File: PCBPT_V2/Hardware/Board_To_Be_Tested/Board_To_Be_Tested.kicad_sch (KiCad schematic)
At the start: 20 parts, among them U1 SHT15, U2 MOUDLE-SEEEDUINO-XIAO

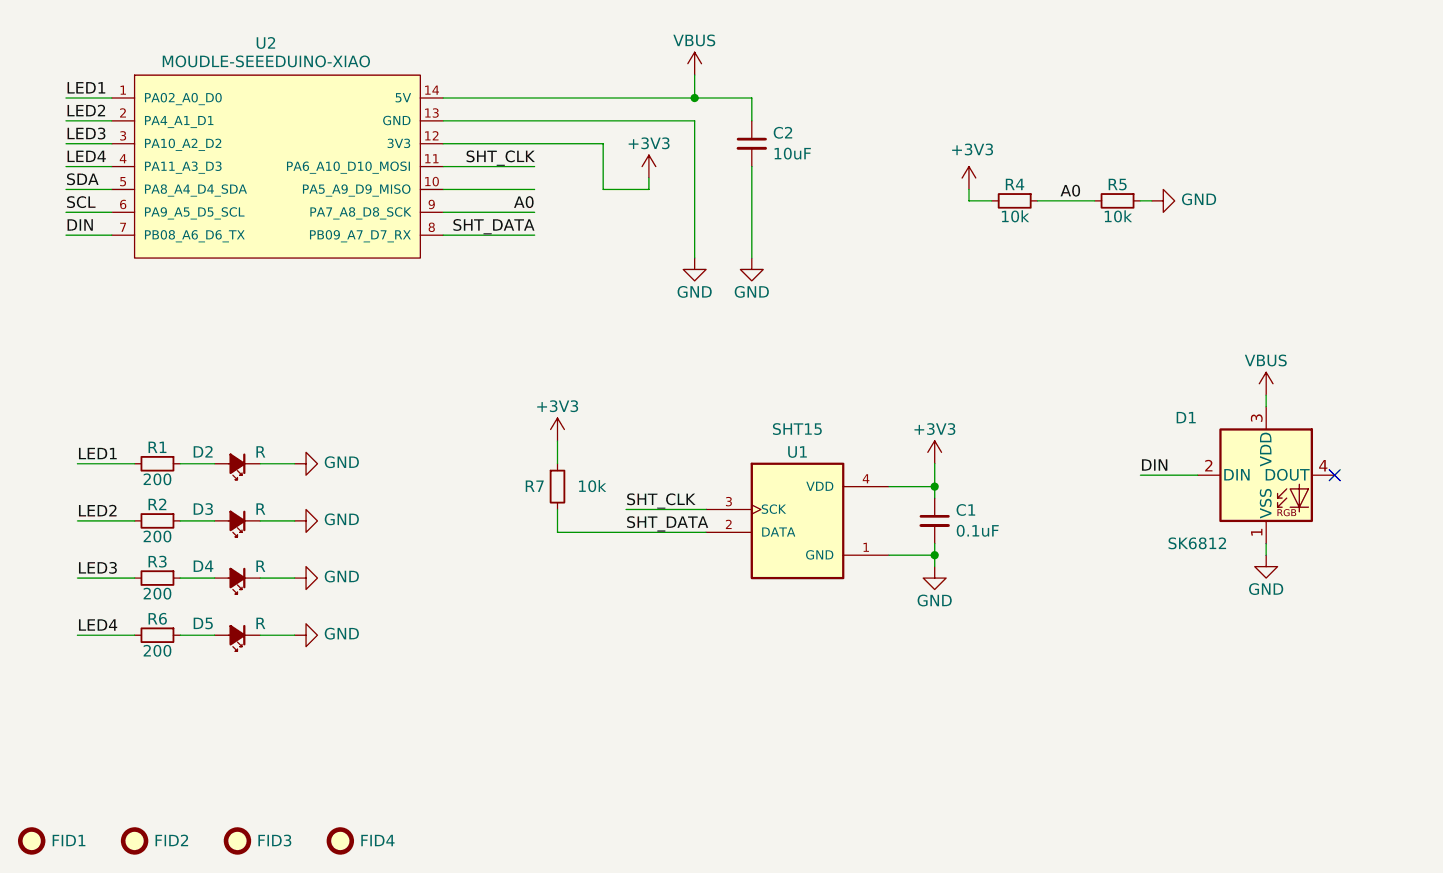
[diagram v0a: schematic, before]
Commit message: udated by FZ
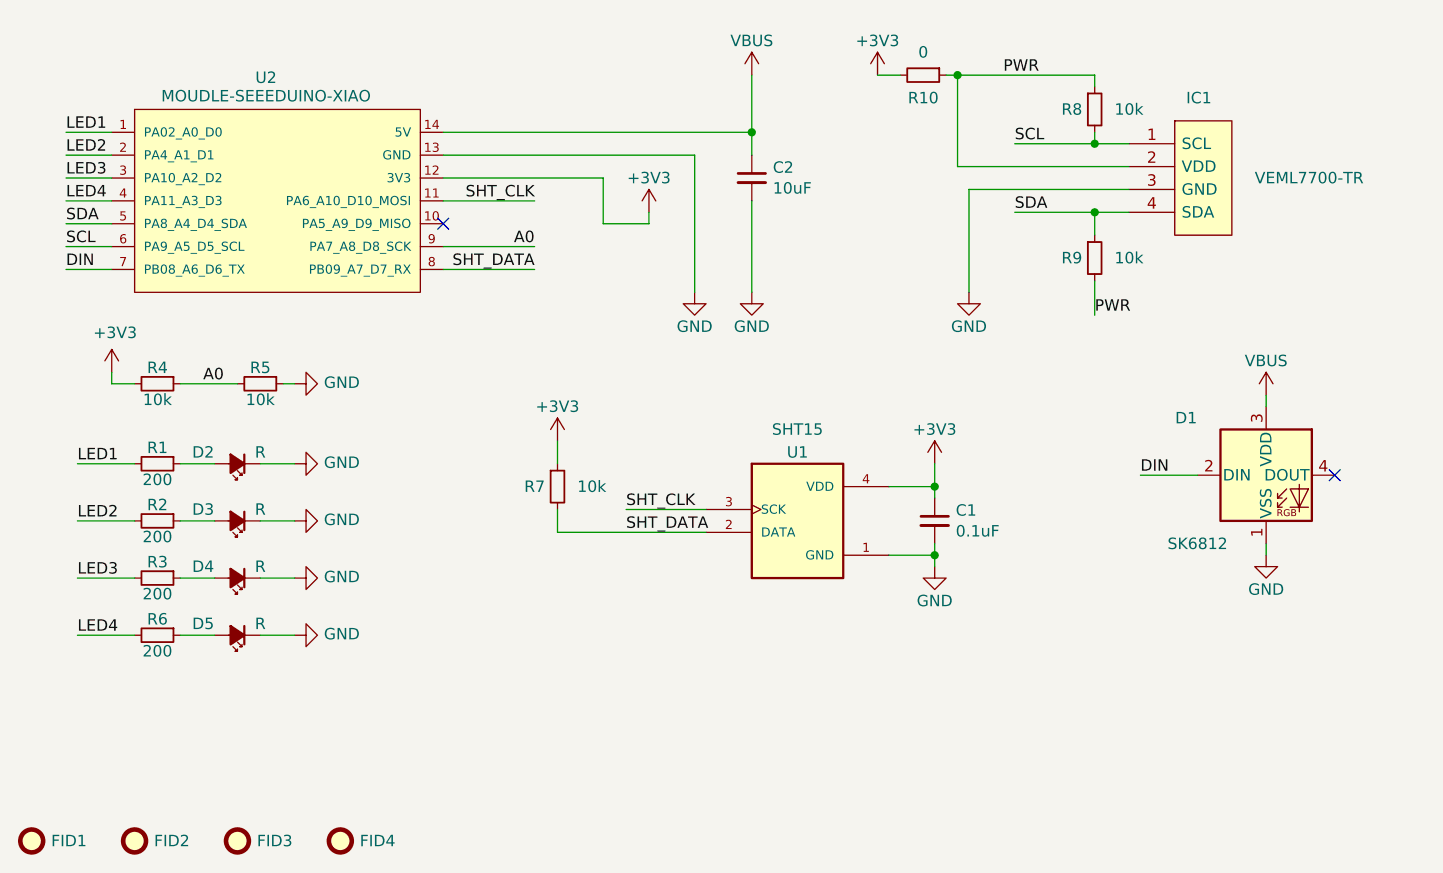
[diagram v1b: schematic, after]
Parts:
- added IC1: VEML7700-TR, SamacSys_Parts:VEML7700, symbol SamacSys_Parts:VEML7700-TR
- added R10: 0, Resistor_SMD:R_1206_3216Metric_Pad1.30x1.75mm_HandSolder, symbol Device:R_Small
- added R8, R9: 10k, Resistor_SMD:R_1206_3216Metric_Pad1.30x1.75mm_HandSolder, symbol Device:R_Small
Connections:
- net +3V3: now also R10.2
- net GND: now also IC1.3 (GND)
- net SCL: now also IC1.1 (SCL), R8.2
- net SDA: now also IC1.4 (SDA), R9.1
- new net PWR: IC1.2 (VDD), R10.1, R8.1, R9.2
- no-connect marks 1 -> 2
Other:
- moved on the sheet: C2, R4, R5, U2

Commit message: udated by FZ
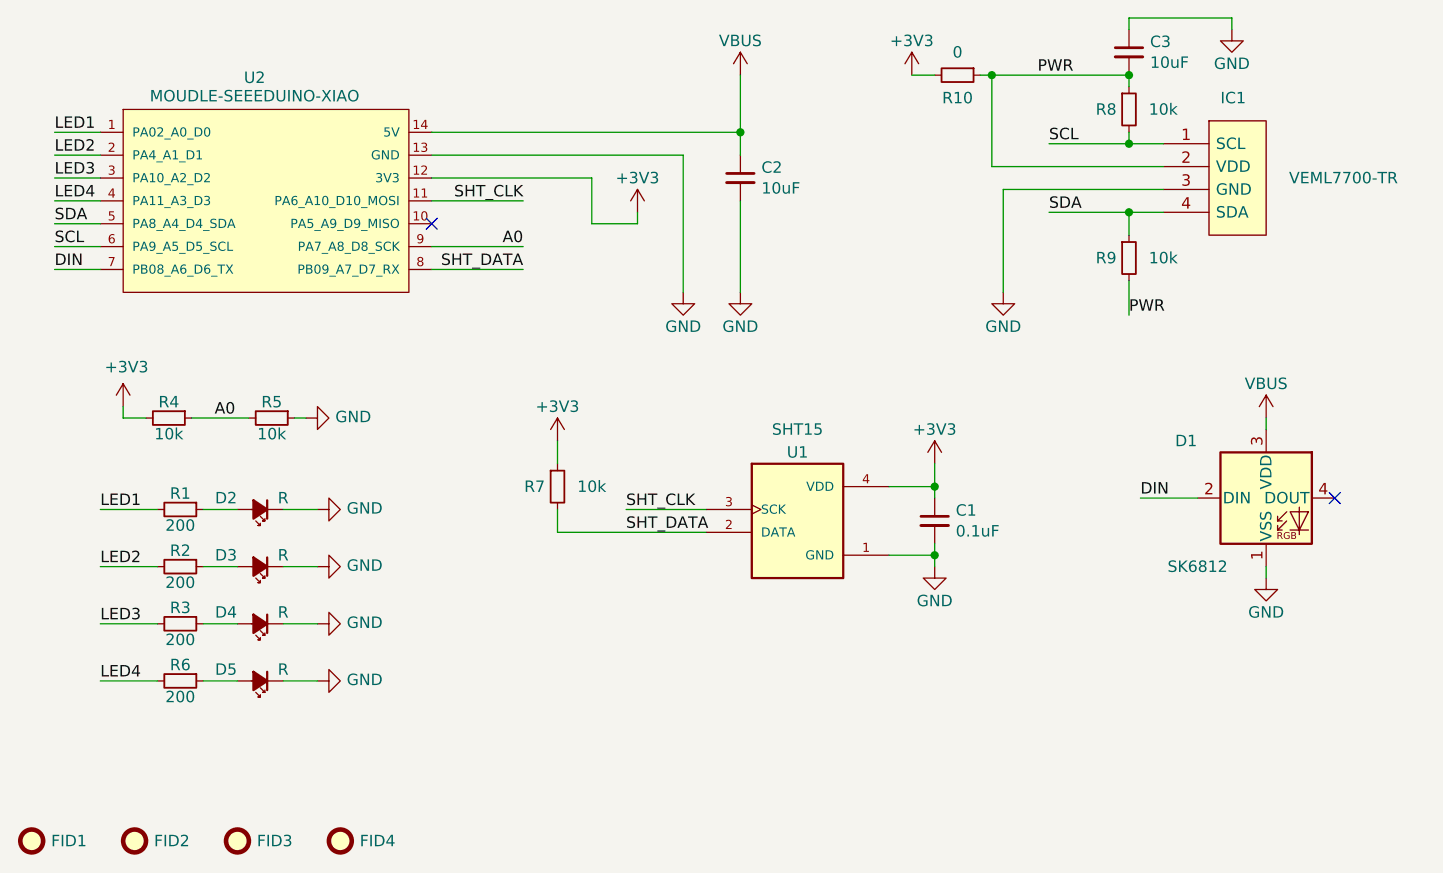
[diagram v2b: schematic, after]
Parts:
- added C3: 10uF, Capacitor_SMD:C_1206_3216Metric_Pad1.33x1.80mm_HandSolder, symbol Device:C_Small
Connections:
- net GND: now also C3.1
- net PWR: now also C3.2
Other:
- moved on the sheet: C2, D1, D2, D3, D4, D5, IC1, R1, R10, R2, R3, R4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
